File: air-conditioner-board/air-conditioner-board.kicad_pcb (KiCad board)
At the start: 2 copper layers, 81.3 x 84.4 mm, 56 parts, among them Q1 BTA16-600BW, U1 DP1801B, U3 EL817, U4 MOC3021M

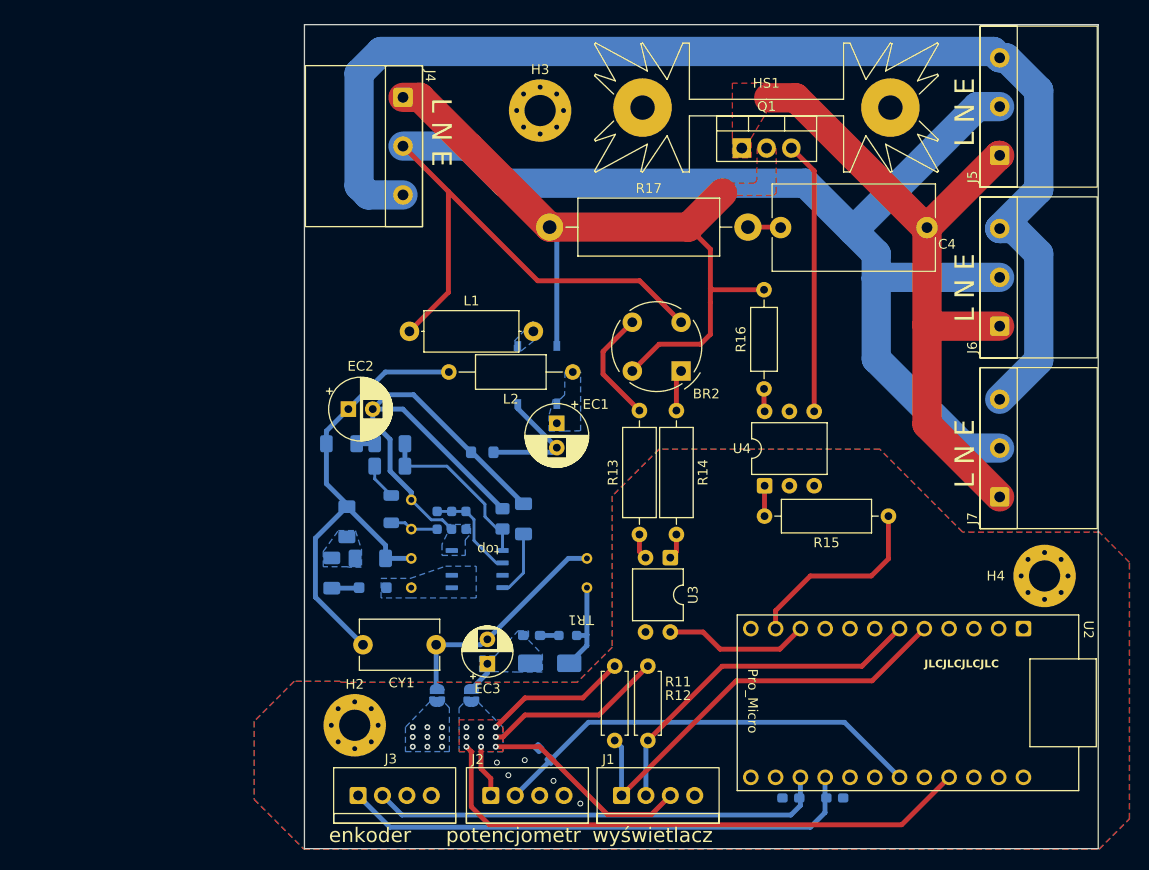
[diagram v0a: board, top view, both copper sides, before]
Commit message: Add layout version 2 - SMPS
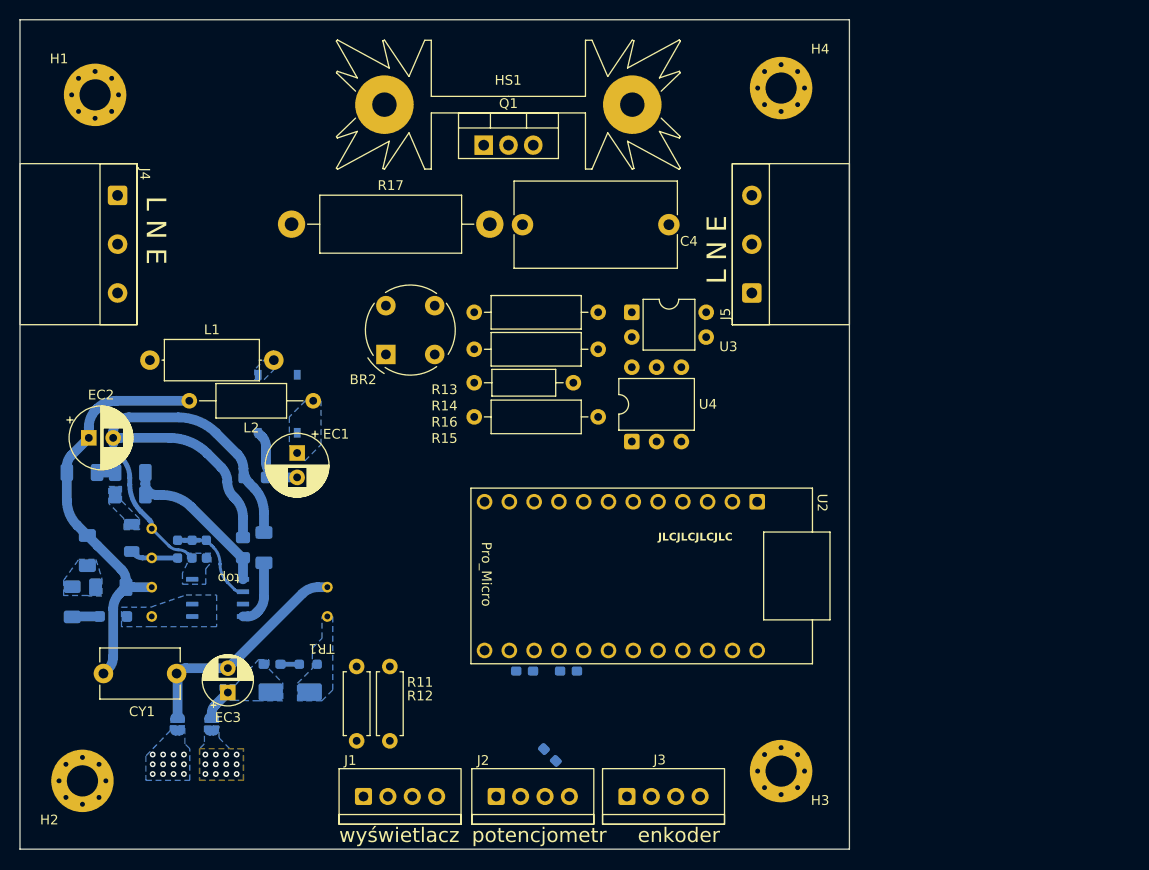
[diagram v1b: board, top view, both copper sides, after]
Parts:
- removed J6, J7: ~, Connector_JOINT_TECH:TBG-5.0-KW-3P
- added H1: MountingHole, MountingHole:MountingHole_3.2mm_M3_Pad_Via, F.Cu at (57.7, 57.7)
- moved H3 72.1 mm to (128.0, 127.0)
- moved H4 56.8 mm to (128.0, 57.0)
- moved R15 43.7 mm to (96.5, 90.7), turned to 0 degrees
- moved J4 30.9 mm to (60.0, 73.0)
- moved BR2 30.3 mm to (87.5, 84.3), turned to 90 degrees
- moved C5 30.2 mm to (101.7, 116.8)
- moved C6 30.2 mm to (106.2, 116.8)
- moved PN1 30.2 mm to (119.2, 103.0)
- moved U2 30.2 mm to (131.2, 98.0)
- moved J5 29.1 mm to (125.0, 73.0)
- moved H2 28.5 mm to (56.4, 128.0)
- moved J3 27.6 mm to (116.0, 129.6)
- moved EC1 26.8 mm to (78.4, 94.4)
- moved BR1 26.8 mm to (76.4, 89.4)
- moved C1 26.8 mm to (59.3, 108.2)
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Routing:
- net NEUTRAL: track 165.2 -> 0.00 mm
- net /output/protection: track 126.1 -> 0.00 mm
- net +5V: track 118.5 -> 0.00 mm, vias 9 -> 12
- net ~230VAC: track 79.3 -> 0.00 mm
- net /output/sterowane wyjście: track 70.4 -> 0.00 mm
- net /MCU/enkoder A: track 53.4 -> 0.00 mm
- net /MCU/enkoder B: track 47.0 -> 0.00 mm
- net /MCU/potencjometr: track 44.8 -> 0.00 mm
- net /MCU/SDA: track 44.0 -> 0.00 mm
- net /MCU/SCL: track 36.3 -> 0.00 mm
- net Net-(Q1-G): track 28.0 -> 0.00 mm
- net /MCU/triac: track 20.0 -> 0.00 mm
- net /MCU/sine sinq: track 14.9 -> 0.00 mm
- net Net-(BR2--): track 11.8 -> 0.00 mm
- net /power/TR1 sec1: track 9.58 -> 0.00 mm
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- added copper zone on B.Cu, net /power/TR1 sec1
- added copper zone on B.Cu, net Net-(D2-Pad1)
- removed copper zone on F.Cu, net /output/sterowane wyjście
- removed copper zone on F.Cu, net GND
- removed copper zone on F.Cu, net ~230VAC
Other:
- board size 81.3 x 84.4 mm -> 85 x 85 mm
